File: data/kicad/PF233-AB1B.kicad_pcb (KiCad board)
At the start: 6 copper layers, 40 x 40 mm, 35 parts, among them J1 Antenna harness 6p solder pad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, J2 Main-board 2x6 1.27mm header, SW1 74LVC1G66, SW2 74LVC1G66, U1 OPA2211

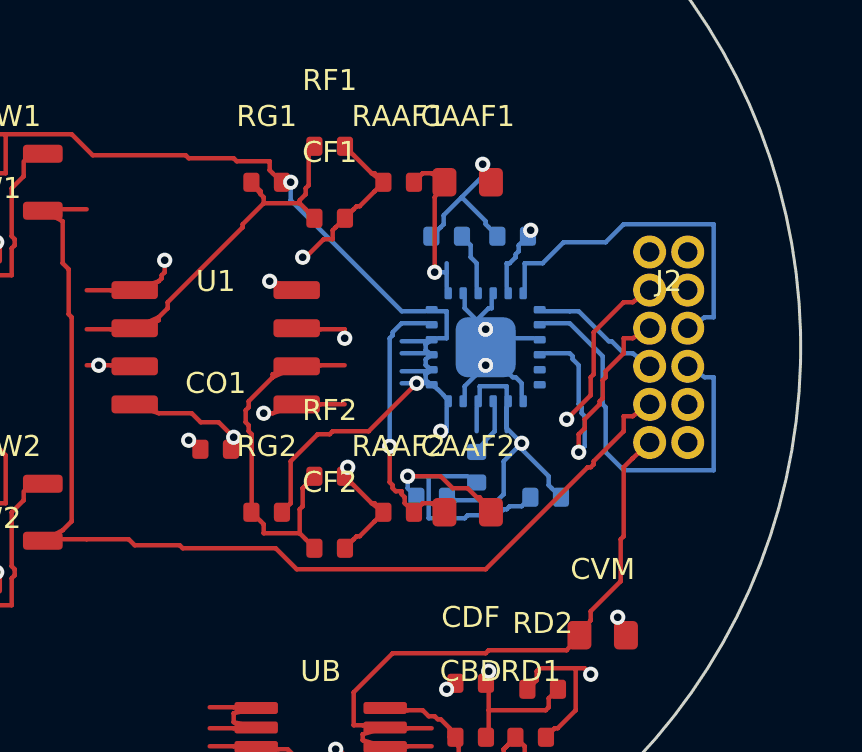
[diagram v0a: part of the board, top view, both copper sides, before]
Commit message: WIP: B5 link check, B6 readout model, B7 datasheets, B8 BOM/PnP + potting + septum lap, B9 rip-up router + drive option, solid_union cache, B3 rows (untested in pipeline)
Co-Authored-By: Claude Opus 5.5 <noreply@anthropic.com>
Claude-Session: https://claude.ai/code/session_01FX4DWSYYjMCFGGA6gmha65
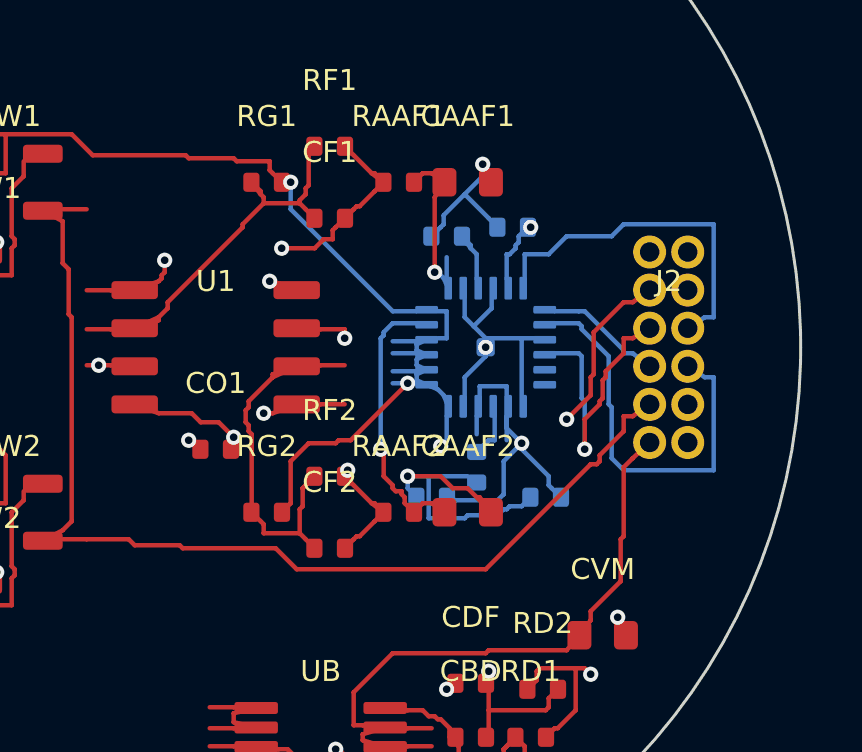
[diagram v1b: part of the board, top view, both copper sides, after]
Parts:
- UA1: footprint Package_CSP:LFCSP-24-1EP_4x4mm_P0.5mm_EP2.65x2.65mm -> Package_CSP:CP-24-25_ADI_LFCSP-24-1EP_4x4mm_P0.5mm_EP0.61x0.61mm
- moved CRF 0.30 mm to (110.4, 96.0)
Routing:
- net GND: track 49.3 -> 50.4 mm, vias 11 -> 10
- net VCM: track 90.3 -> 91.2 mm
